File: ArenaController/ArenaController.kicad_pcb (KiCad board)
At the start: 2 copper layers, 63 x 112.3 mm, 34 parts, among them J1 RJ45, J2 RJ45, J4 RJ45, J5 RJ45, J6 RJ45, J8 Screw_Terminal_01x04, J9 Barrel_Jack_MountingPin, Q1 FS3400, Q2 FS3400, Q3 FS3400, Q4 FS3400, Q5 FS3400, Q6 Q_NMOS_GSD, U3 ESP32-Devkit_C_V4

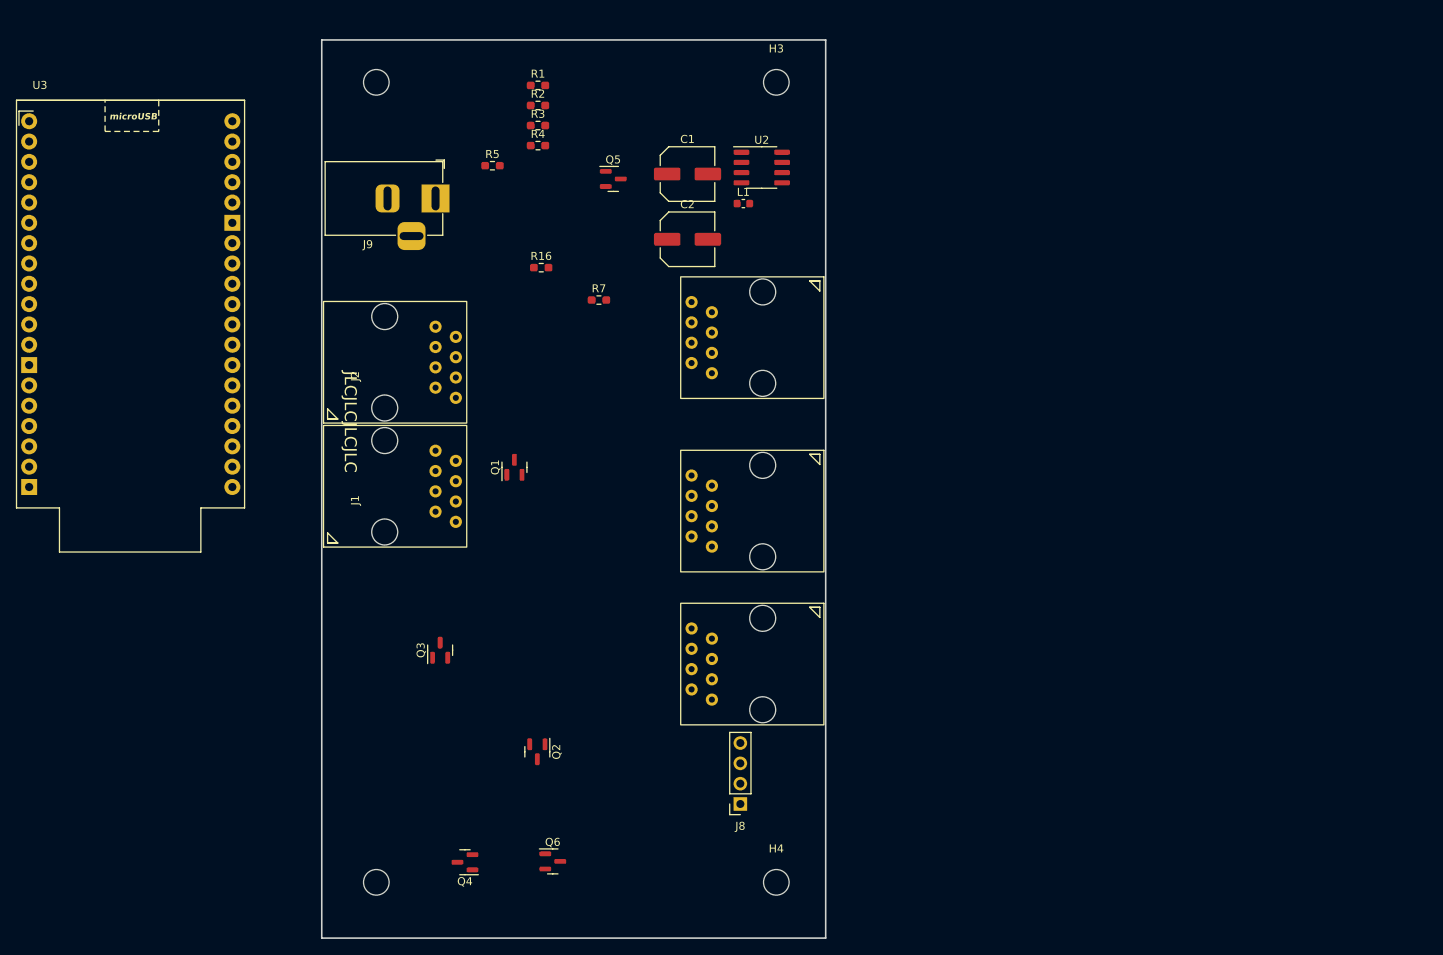
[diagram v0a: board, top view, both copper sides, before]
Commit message: small boardwork cleanup to try and lay it out.
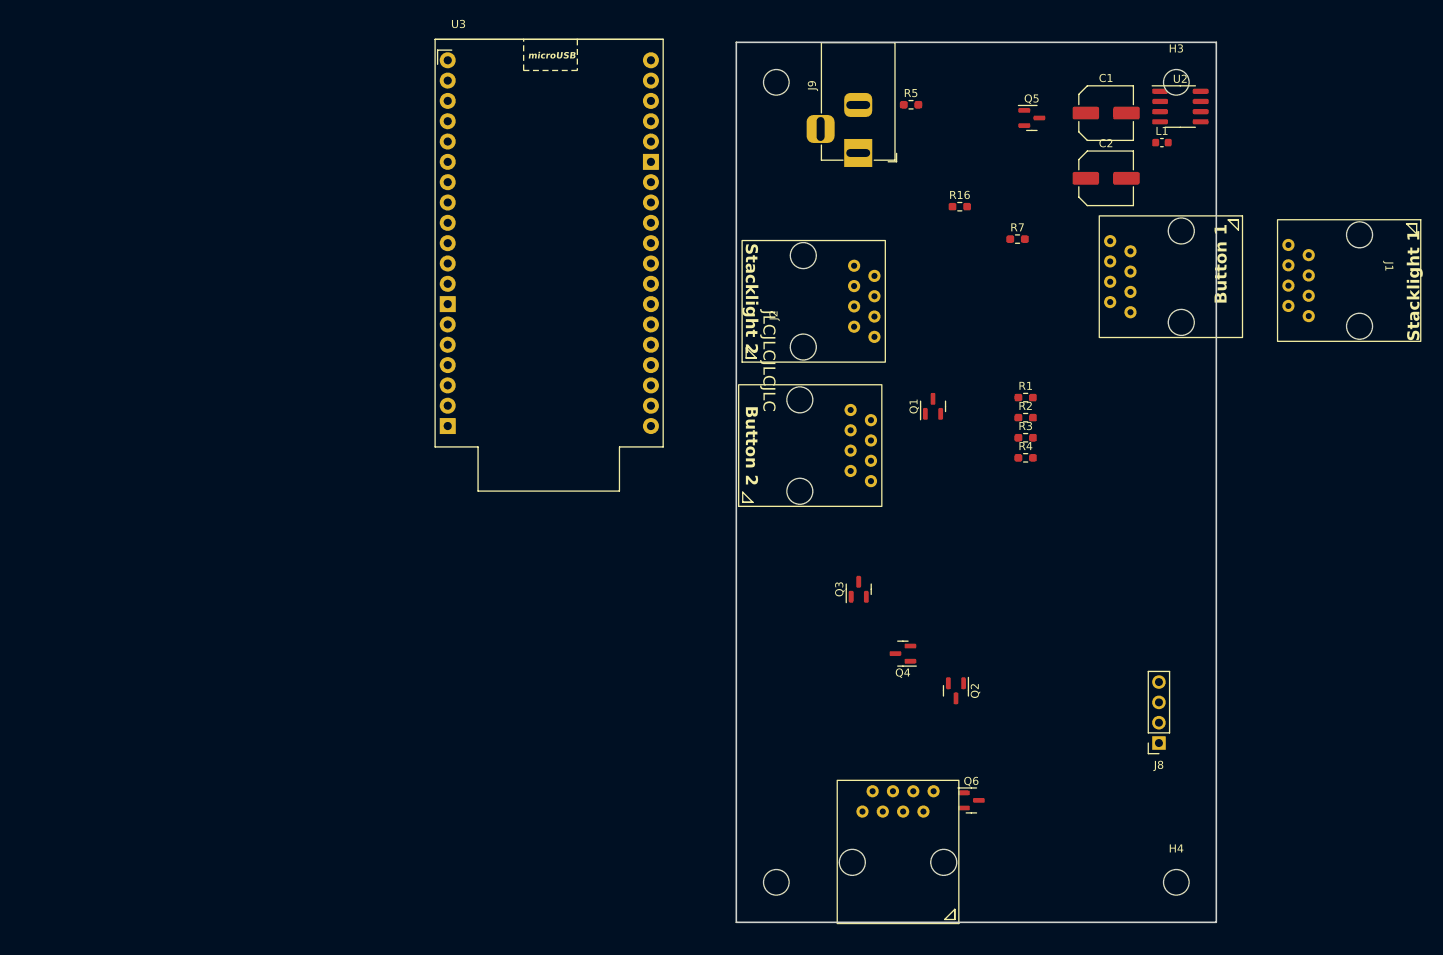
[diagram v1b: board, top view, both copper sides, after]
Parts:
- removed kibuzzard-638A2138: G***, kibuzzard-638A2138
- removed kibuzzard-638A214B: G***, kibuzzard-638A214B
- removed kibuzzard-638A2165: G***, kibuzzard-638A2165
- removed kibuzzard-638A2178: G***, kibuzzard-638A2178
- moved J1 143.1 mm to (180.6, 67.2), turned to -90 degrees
- moved R1 72.4 mm to (131.2, 89.4)
- moved R2 72.4 mm to (131.2, 91.9)
- moved R3 72.4 mm to (131.2, 94.4)
- moved R4 72.4 mm to (131.2, 96.9)
- moved J4 61.5 mm to (122.8, 155.2), turned to 180 degrees
- moved Q4 60.6 mm to (115.8, 121.4)
- moved J9 53.1 mm to (110.2, 58.8), turned to -90 degrees
- moved L1 52.9 mm to (148.2, 57.5)
- moved R16 52.9 mm to (122.9, 65.5)
- moved Q3 52.9 mm to (110.3, 113.4)
- moved J6 52.9 mm to (158.3, 66.7)
- moved J8 52.9 mm to (147.8, 132.6)
- moved Q1 52.9 mm to (119.6, 90.5)
- moved Q2 52.9 mm to (122.5, 126.1)
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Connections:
- J4 pad 5: /G_Pause -> unconnected-(J4-Pad5)
- J4 pad 6: /G_End -> unconnected-(J4-Pad6)
- J4 pad 7: /G_Reset -> /G_End
- U2 pad 2: (no net) -> unconnected-(U2-NC-Pad2)
- U3 pad 11: /G_Reset -> unconnected-(U3-GPIO18/V_SPI_CLK/SCK-Pad11)
- U3 pad 25: /G_Pause -> unconnected-(U3-RTC_GPIO5/ADC1_7/GPIO35-Pad25)
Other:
- board size 63 x 112.3 mm -> 60 x 110 mm
- board text added: "Button 1"
- board text added: "Button 2"
- board text added: "Stacklight 1"
- board text added: "Stacklight 2"
